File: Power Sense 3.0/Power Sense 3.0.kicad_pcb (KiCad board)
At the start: 2 copper layers, 133.9 x 50.3 mm, 49 parts, among them IC1 MCP3909, J1 Power, J2 ProgHead, J3 SPI, J4 TestHeader, T1 AC1030, T2 2p2sTransformer, U1 PIC18F25K20_I/SS, Y1 3.579545MHz Crystal

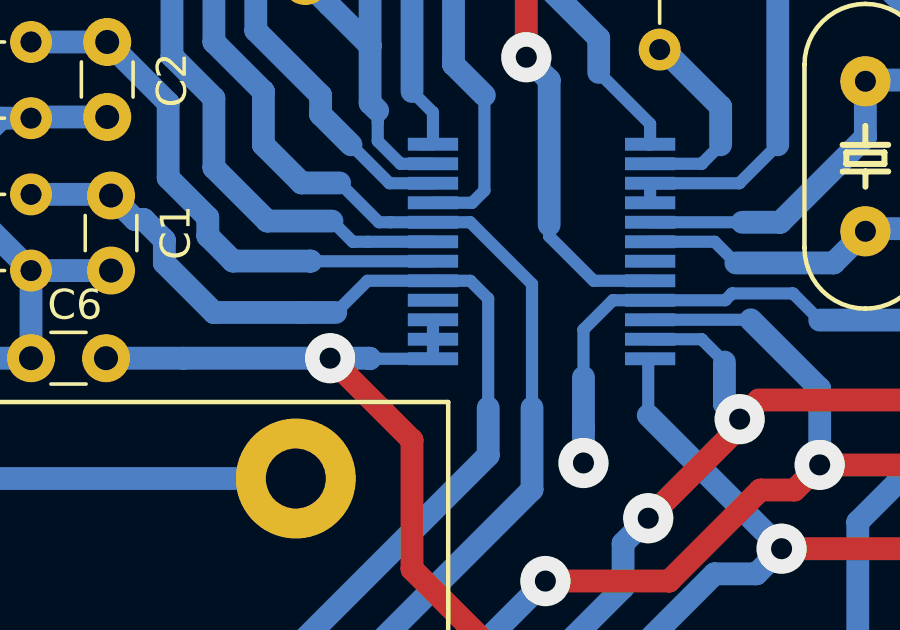
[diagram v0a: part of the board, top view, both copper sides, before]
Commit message: First round of edits
Edited things in README.txt
See that file for changes
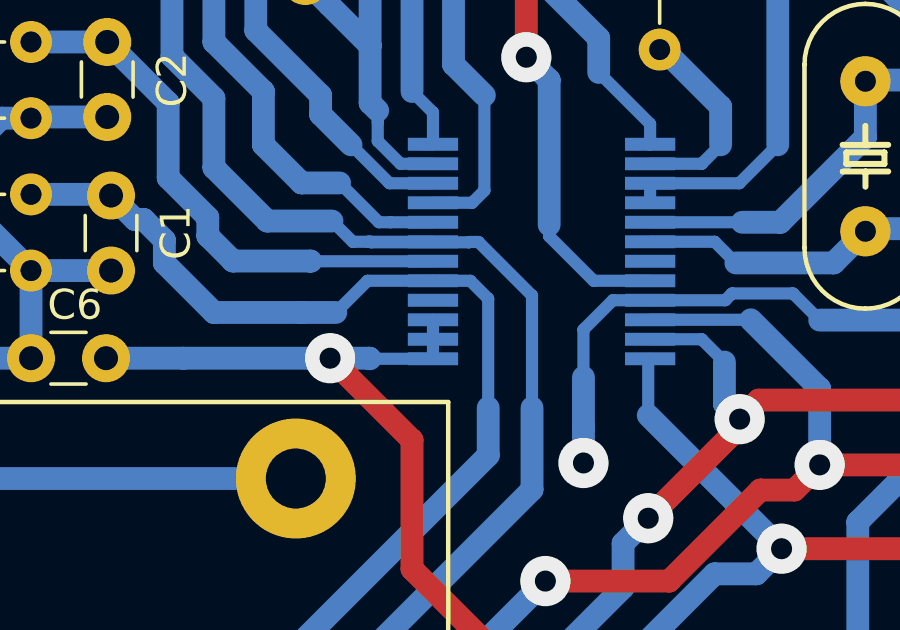
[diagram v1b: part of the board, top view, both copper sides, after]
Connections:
- C3 pad 2: Net-(C3-Pad2) -> /CH1-
- IC1 pad 7: Net-(C3-Pad2) -> /CH1-
- J4 pad 4: /CH1+ -> /CH1-
- R8 pad 2: Net-(C3-Pad2) -> /CH1-
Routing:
- net /CH1-: track 0.00 -> 52.6 mm
- net /CH1+: track 58.3 -> 29.7 mm
- net Net-(C3-Pad2): track 22.3 -> 0.00 mm
- net GND: track 295.8 -> 300.6 mm, vias 7 -> 8
- net (no net): track 9.70 -> 4.87 mm, vias 1 -> 0
